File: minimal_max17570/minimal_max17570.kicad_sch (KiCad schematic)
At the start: 0 parts

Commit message: backup
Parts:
- added C1: 1 µF, capacitor_footprints:C_0402_1005Metric, symbol CAPACITORS_C1005X6S1C_DATA_BASE:C_C1005X6S1C105K050BC
- added C2: 10 µF, capacitor_footprints:C_1206_3216Metric, symbol CAPACITORS_CL31B_DATA_BASE:C_CL31B106KBHNNN#
- added C3: 1 µF, capacitor_footprints:C_0805_2012Metric, symbol CAPACITORS_GRJ21BC72A_DATA_BASE:C_GRJ21BC72A105KE11L
- added L1: 100.0 µH, inductor_footprints:74404054, symbol INDUCTORS_74404054_DATA_BASE:L_74404054101
- added R1: 40.2 kΩ, resistor_footprints:R_0402_1005Metric, symbol RESISTORS_ERJ-2RKF_DATA_BASE:R_ERJ-2RKF4022X
- added R2: 9.76 kΩ, resistor_footprints:R_0402_1005Metric, symbol RESISTORS_ERJ-2RKF_DATA_BASE:R_ERJ-2RKF9761X
- added R3: 499 kΩ, resistor_footprints:R_0402_1005Metric, symbol RESISTORS_ERJ-2RKF_DATA_BASE:R_ERJ-2RKF4993X
- added R4: 1 kΩ, resistor_footprints:R_0402_1005Metric, symbol UNITED_RESISTORS_DATA_BASE:R_ERJ-2RKF1001X
- added R5: 3.32 MΩ, resistor_footprints:R_0402_1005Metric, symbol RESISTORS_RC0402FR-07_DATA_BASE:R_RC0402FR-073M32L
- added R6: 294 kΩ, resistor_footprints:R_0402_1005Metric, symbol RESISTORS_ERJ-2RKF_DATA_BASE:R_ERJ-2RKF2943X
- added U1: MAX17570FATA+, analog_devices_footprints:21-100514_T822C&plus_6C_ADI, symbol UNITED_IC_ADI:U_MAX17570FATA+
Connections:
- new net: R2.1, U1.5 (RT/SYNC)
- new net EN: R5.2, R6.1, U1.2 (EN/UVLO)
- new net FB: R1.1, R3.2, U1.4 (VOUT/FB)
- new net GND: C1.2, C2.2, C3.2, R1.2, R2.2, R6.2, U1.7 (GND)
- new net LX: L1.1, U1.8 (LX)
- new net VCC: C1.1, R4.1, U1.3 (VCC)
- new net VIN: C3.1, R5.1, U1.1 (VIN)
- new net VOUT: C2.1, L1.2, R3.1
- new net ~{RESET}: R4.2, U1.6 (~{RESET})

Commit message: backup
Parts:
- R4: symbol UNITED_RESISTORS_DATA_BASE:R_ERJ-2RKF1001X -> RESISTORS_ERJ-2RKF_DATA_BASE:R_ERJ-2RKF1001X
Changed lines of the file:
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@@
 		(dnp no)
 		(fields_autoplaced yes)
-		(property "Reference" "#PWR02"
+		(property "Reference" "#PWR2"
 			(at 203.2 97.79 0)
 			(effects
@@
 			(project "minimal_max17570"
 				(path "/92f3cd93-efd9-4305-a902-cde57c556096"
-					(reference "#PWR02")
+					(reference "#PWR2")
 					(unit 1)
 				)
@@
 		(dnp no)
 		(fields_autoplaced yes)
-		(property "Reference" "#PWR04"
+		(property "Reference" "#PWR4"
 			(at 190.5 118.11 0)
 			(effects
@@
 			(project "minimal_max17570"
 				(path "/92f3cd93-efd9-4305-a902-cde57c556096"
-					(reference "#PWR04")
+					(reference "#PWR4")
 					(unit 1)
 				)
@@
 		(dnp no)
 		(fields_autoplaced yes)
-		(property "Reference" "#PWR06"
+		(property "Reference" "#PWR6"
 			(at 111.76 97.79 0)
 			(effects
@@
 			(project "minimal_max17570"
 				(path "/92f3cd93-efd9-4305-a902-cde57c556096"
-					(reference "#PWR06")
+					(reference "#PWR6")
 					(unit 1)
 				)
@@
 	)
 	(symbol
-		(lib_id "UNITED_RESISTORS_DATA_BASE:R_ERJ-2RKF1001X")
+		(lib_id "RESISTORS_ERJ-2RKF_DATA_BASE:R_ERJ-2RKF1001X")
 		(at 170.18 110.49 90)
 		(mirror x)
@@
 		(dnp no)
 		(fields_autoplaced yes)
-		(property "Reference" "#PWR03"
+		(property "Reference" "#PWR3"
 			(at 134.62 135.89 0)
 			(effects
@@
 			(project "minimal_max17570"
 				(path "/92f3cd93-efd9-4305-a902-cde57c556096"
-					(reference "#PWR03")
+					(reference "#PWR3")
 					(unit 1)
 				)
@@
 		(dnp no)
 		(fields_autoplaced yes)
-		(property "Reference" "#PWR07"
+		(property "Reference" "#PWR7"
 			(at 127 118.11 0)
 			(effects
@@
 			(project "minimal_max17570"
 				(path "/92f3cd93-efd9-4305-a902-cde57c556096"
-					(reference "#PWR07")
+					(reference "#PWR7")
 					(unit 1)
 				)
@@
 		(dnp no)
 		(fields_autoplaced yes)
-		(property "Reference" "#PWR01"
+		(property "Reference" "#PWR1"
 			(at 152.4 129.54 0)
 			(effects
@@
 			(project ""
 				(path "/92f3cd93-efd9-4305-a902-cde57c556096"
-					(reference "#PWR01")
+					(reference "#PWR1")
 					(unit 1)
 				)
@@
 		(dnp no)
 		(fields_autoplaced yes)
-		(property "Reference" "#PWR05"
+		(property "Reference" "#PWR5"
 			(at 162.56 78.74 0)
 			(effects
@@
 			(project "minimal_max17570"
 				(path "/92f3cd93-efd9-4305-a902-cde57c556096"
-					(reference "#PWR05")
+					(reference "#PWR5")
 					(unit 1)
 				)

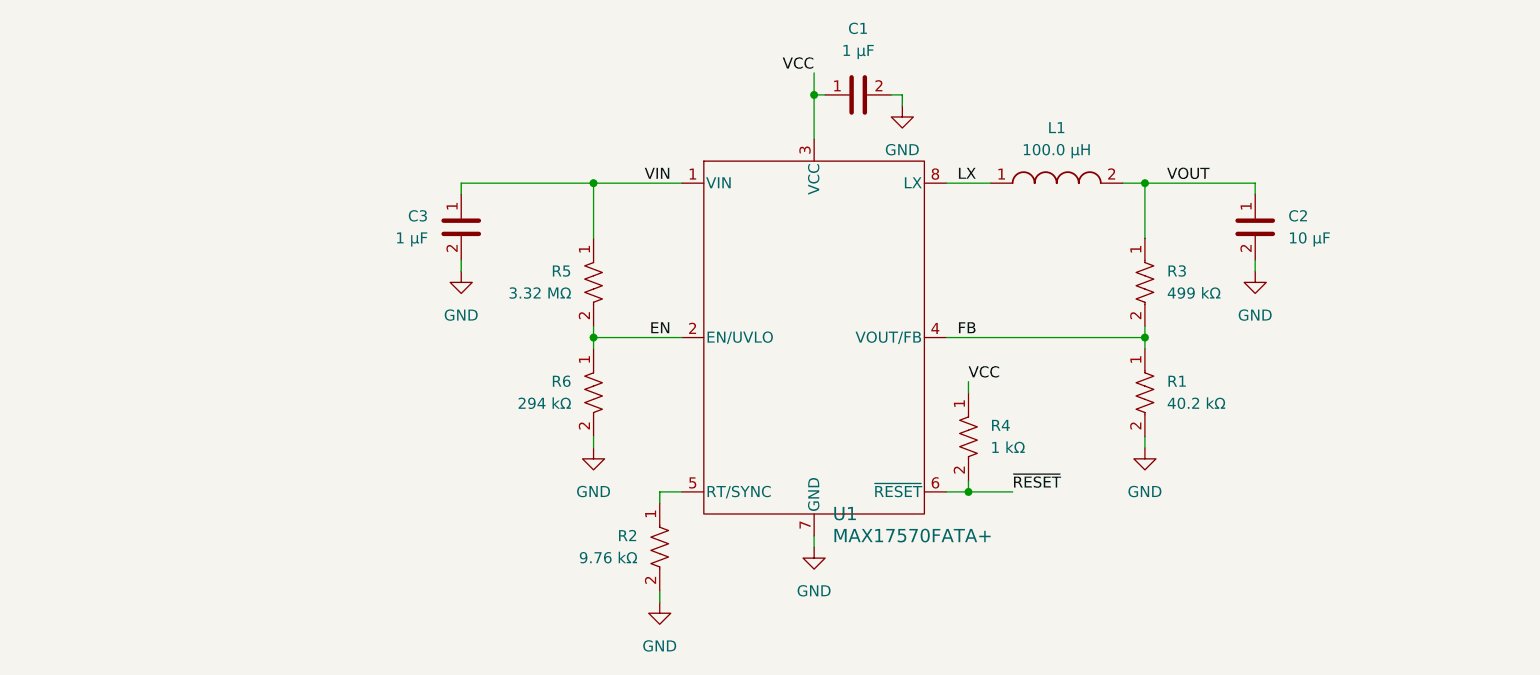
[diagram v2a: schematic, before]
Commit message: backup
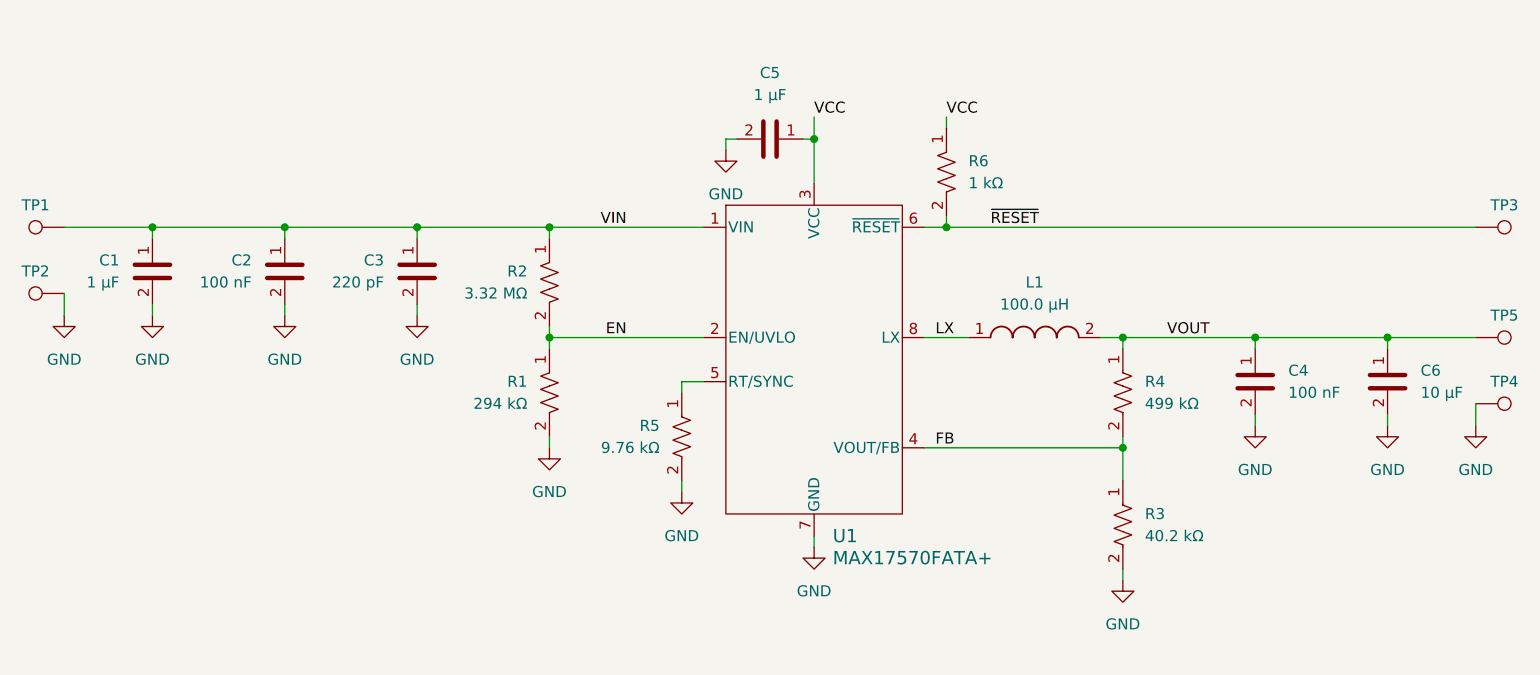
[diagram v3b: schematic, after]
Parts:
- added C2, C4: 100 nF, capacitor_footprints:C_0603_1608Metric, symbol CAPACITORS_C1608X7S2A_DATA_BASE:C_C1608X7S2A104K080AB
- added C3: 220 pF, capacitor_footprints:C_0402_1005Metric, symbol CAPACITORS_CGA2B2NP02A_DATA_BASE:C_CGA2B2NP02A221J050BA
- added TP1, TP2, TP3, TP4, TP5: TestPoint, test_point_footprints:TestPoint_THTPad_Castelated, symbol UNITED_TEST_POINTS:TestPoint_Castelated
- renumbered C3 to C1, C1 to C5, C2 to C6, R6 to R1, R5 to R2, R1 to R3, R3 to R4, R2 to R5, R4 to R6
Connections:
- net GND: now also C2.2, C3.2, C4.2, TP2.1, TP4.1
- net VIN: now also C2.1, C3.1, TP1.1
- net VOUT: now also C4.1, TP5.1
- net ~{RESET}: now also TP3.1
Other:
- moved on the sheet: C1, C5, C6, L1, R1, R2, R3, R4, R5, R6, U1
